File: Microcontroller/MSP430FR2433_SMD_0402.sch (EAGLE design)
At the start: 11 parts, among them IC2 MSP430FR2433IRGET, Q1 32.768

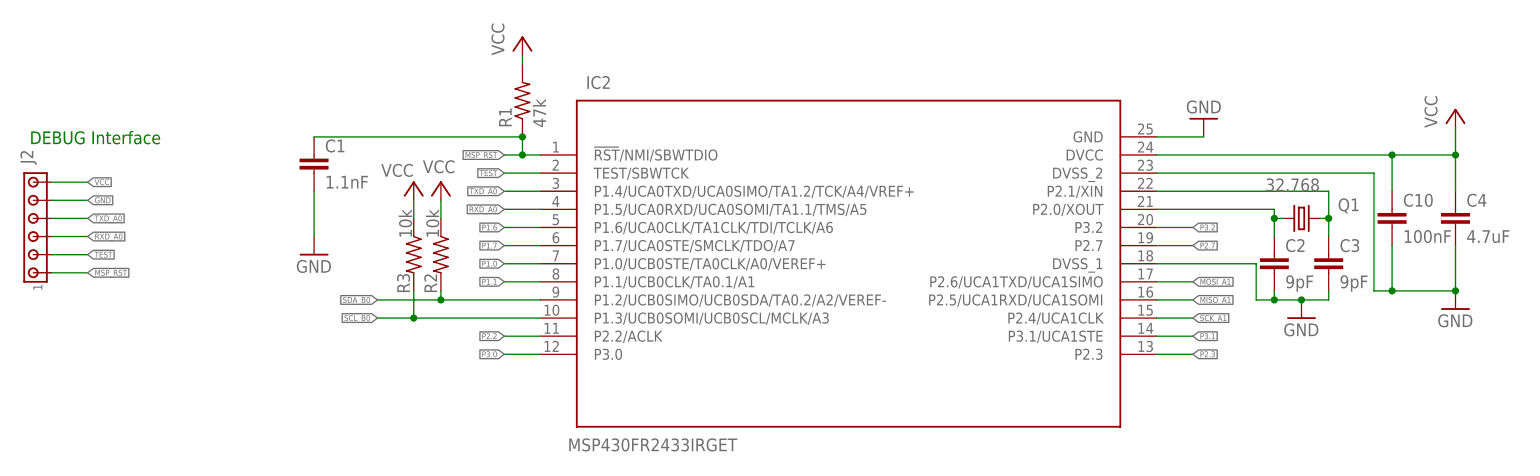
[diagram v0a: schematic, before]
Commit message: updated lot of ckt
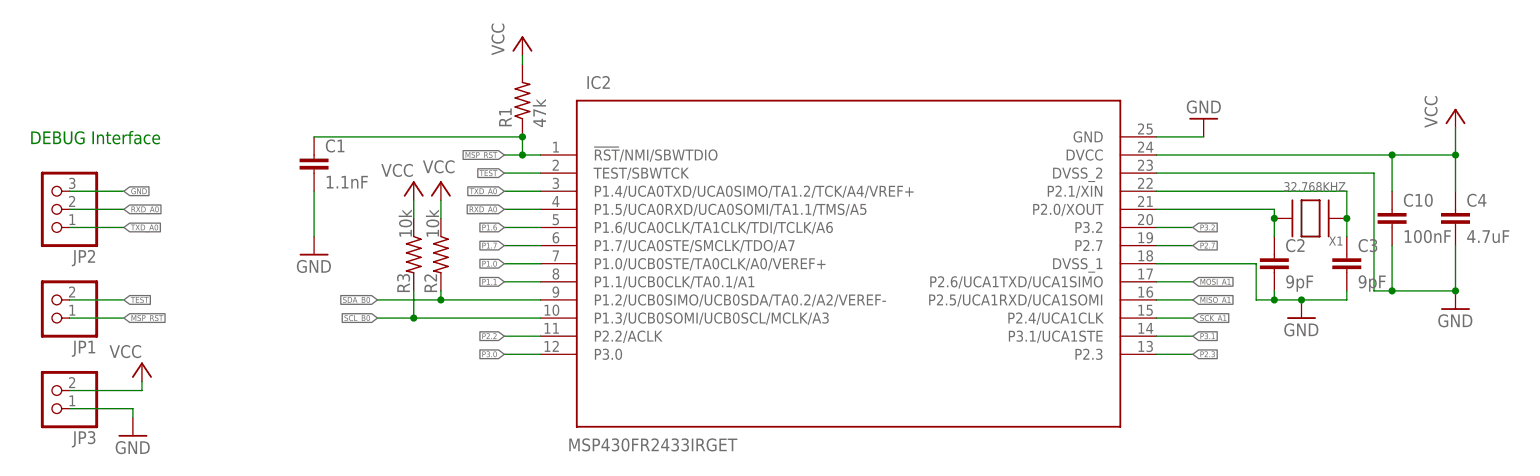
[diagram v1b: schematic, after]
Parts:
- removed J2: (no value), con-amp:MTA06-100
- removed Q1: 32.768, crystal:CRYTALTC26H
- added JP1, JP3: (no value), pinhead:PINHD-1X2
- added JP2: (no value), pinhead:PINHD-1X3
- added X1: 32.768KHZ, adafruit:XTAL-3.2X1.5
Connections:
- net GND: now also JP2.3, JP3.1; no longer J2.5
- net MSP_RST: now also JP1.1; no longer J2.1
- net N$1: now also X1.P$1; no longer Q1.1
- net N$3: now also X1.P$2; no longer Q1.2
- net RXD_A0: now also JP2.2; no longer J2.3
- net TEST: now also JP1.2; no longer J2.2
- net TXD_A0: now also JP2.1; no longer J2.4
- net VCC: now also JP3.2; no longer J2.6
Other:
- moved on the sheet: C3
